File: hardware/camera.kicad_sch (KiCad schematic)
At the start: 4 parts, among them J1 524352271

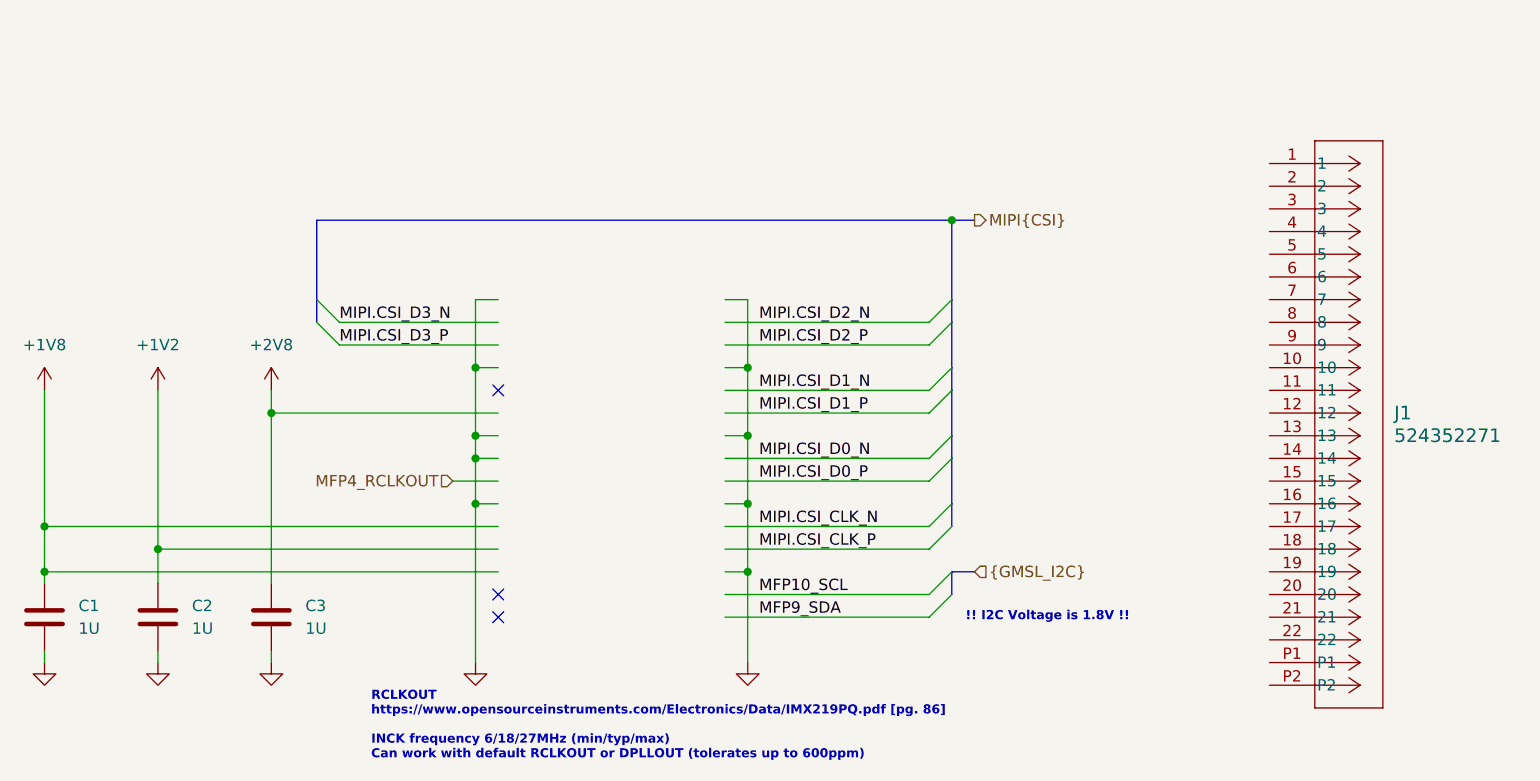
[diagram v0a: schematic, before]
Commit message: cleaned up schematics
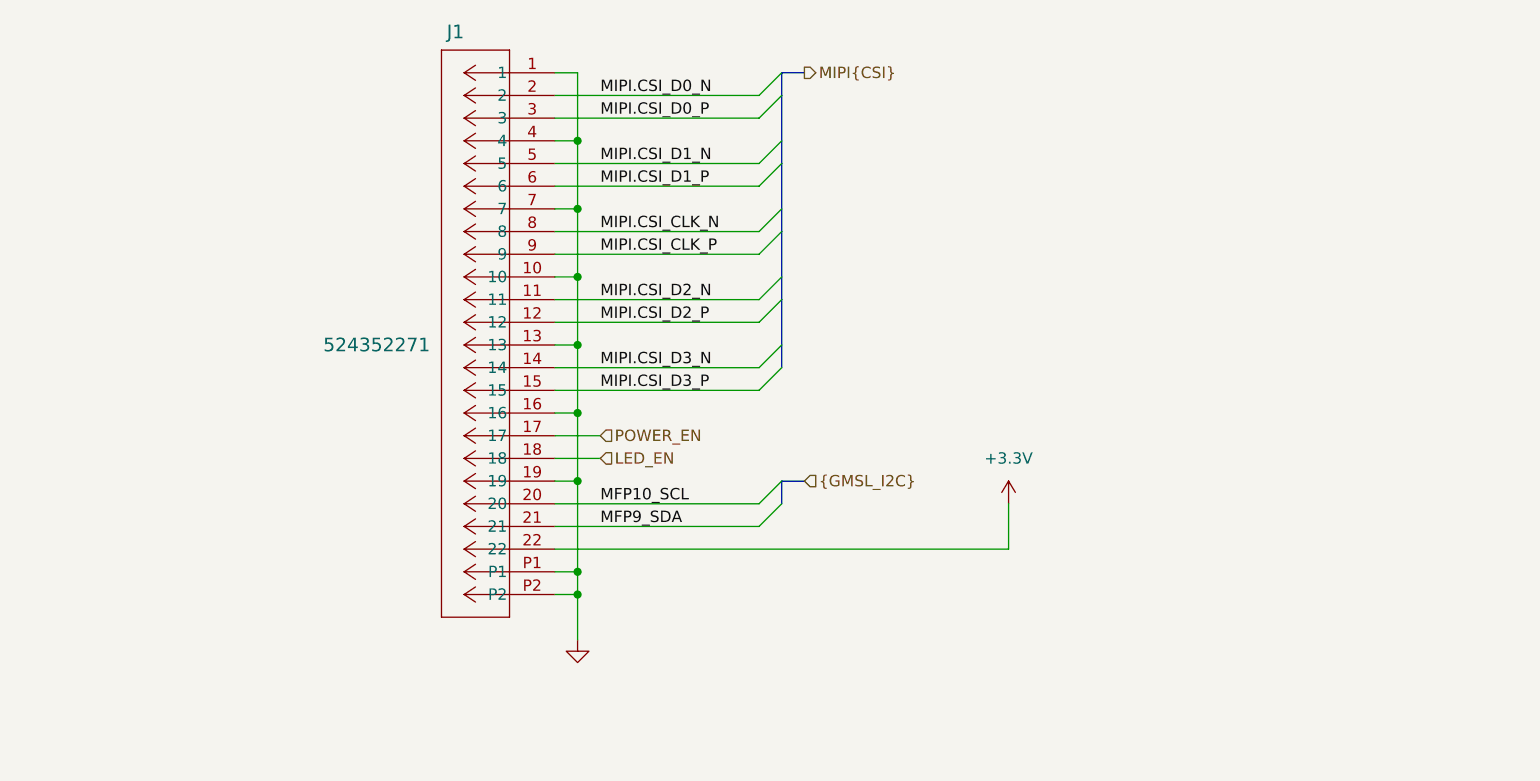
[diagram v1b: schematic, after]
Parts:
- removed C1, C2, C3: 1U, Capacitor_SMD:C_0402_1005Metric, symbol Device:C
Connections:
- net GND: now also J1.1, J1.10, J1.13, J1.16, J1.19, J1.4, J1.7, J1.P1, J1.P2
- net MFP10_SCL: now also J1.20
- net MFP9_SDA: now also J1.21
- net MIPI.CSI_CLK_N: now also J1.8
- net MIPI.CSI_CLK_P: now also J1.9
- net MIPI.CSI_D0_N: now also J1.2
- net MIPI.CSI_D0_P: now also J1.3
- net MIPI.CSI_D1_N: now also J1.5
- net MIPI.CSI_D1_P: now also J1.6
- net MIPI.CSI_D2_N: now also J1.11
- net MIPI.CSI_D2_P: now also J1.12
- net MIPI.CSI_D3_N: now also J1.14
- net MIPI.CSI_D3_P: now also J1.15
- net POWER_EN: now reaches J1.17
- net LED_EN: now reaches J1.18
- net +3.3V: now reaches J1.22
- no-connect marks 3 -> 0
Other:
- note removed: "!! I2C Voltage is 1.8V !!"
- note removed: "RCLKOUT https://www.opensourceinstruments.com/Electronics/Data/IMX219PQ.pdf [pg. 86] INCK frequency 6/18/27MHz (min/typ/max) Can work with default RCLKOUT or DPLLOUT (tolerates up to 600ppm)"
- moved on the sheet: J1
